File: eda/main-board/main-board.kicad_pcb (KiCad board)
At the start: 2 copper layers, 64 parts, among them J1 RomHighSel, J2 Membank block, J3 Expansion, J4 $1-3 latch, J5 PWR, J6 CS_leds, U1 W65C02SxP, U10 74HCT00, U11 74HCT32, U12 74HCT32, U13 74HCT138, U14 74LHCT157, U15 74LHCT157, U16 74HCT273, U2 NA555P, U3 28C256, U4 AS6C4008-55PCN, U5 74HCT138, U6 74HCT32, U7 74HCT08, U8 74HCT30, U9 74HCT139, X1 4Mhz

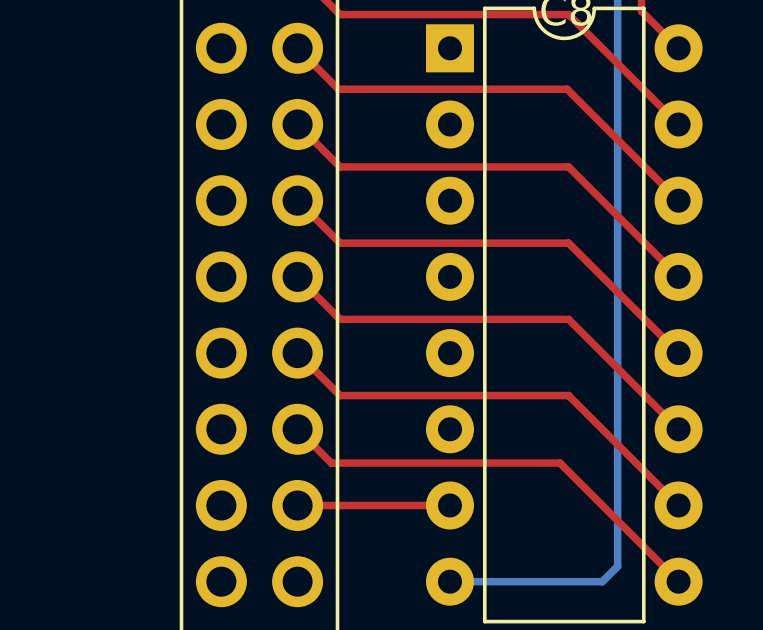
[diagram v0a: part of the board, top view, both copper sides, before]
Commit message: Update eda
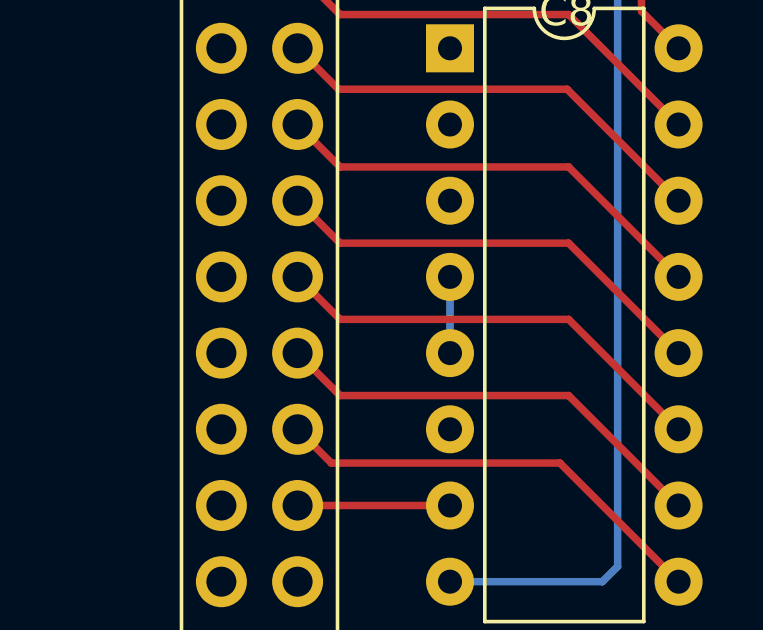
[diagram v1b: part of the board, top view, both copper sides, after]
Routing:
- net /Address decode/~{Io1Cs}: track 0.00 -> 2.54 mm
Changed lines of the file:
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@@
   (segment (start 269.748 146.812) (end 270.873 147.937) (width 0.25) (layer "F.Cu") (net 63))
   (segment (start 274.828 149.352) (end 269.748 149.352) (width 0.25) (layer "F.Cu") (net 64))
+  (segment (start 274.828 144.272) (end 274.828 141.732) (width 0.25) (layer "B.Cu") (net 77))
 )
